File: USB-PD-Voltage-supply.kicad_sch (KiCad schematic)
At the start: 0 parts

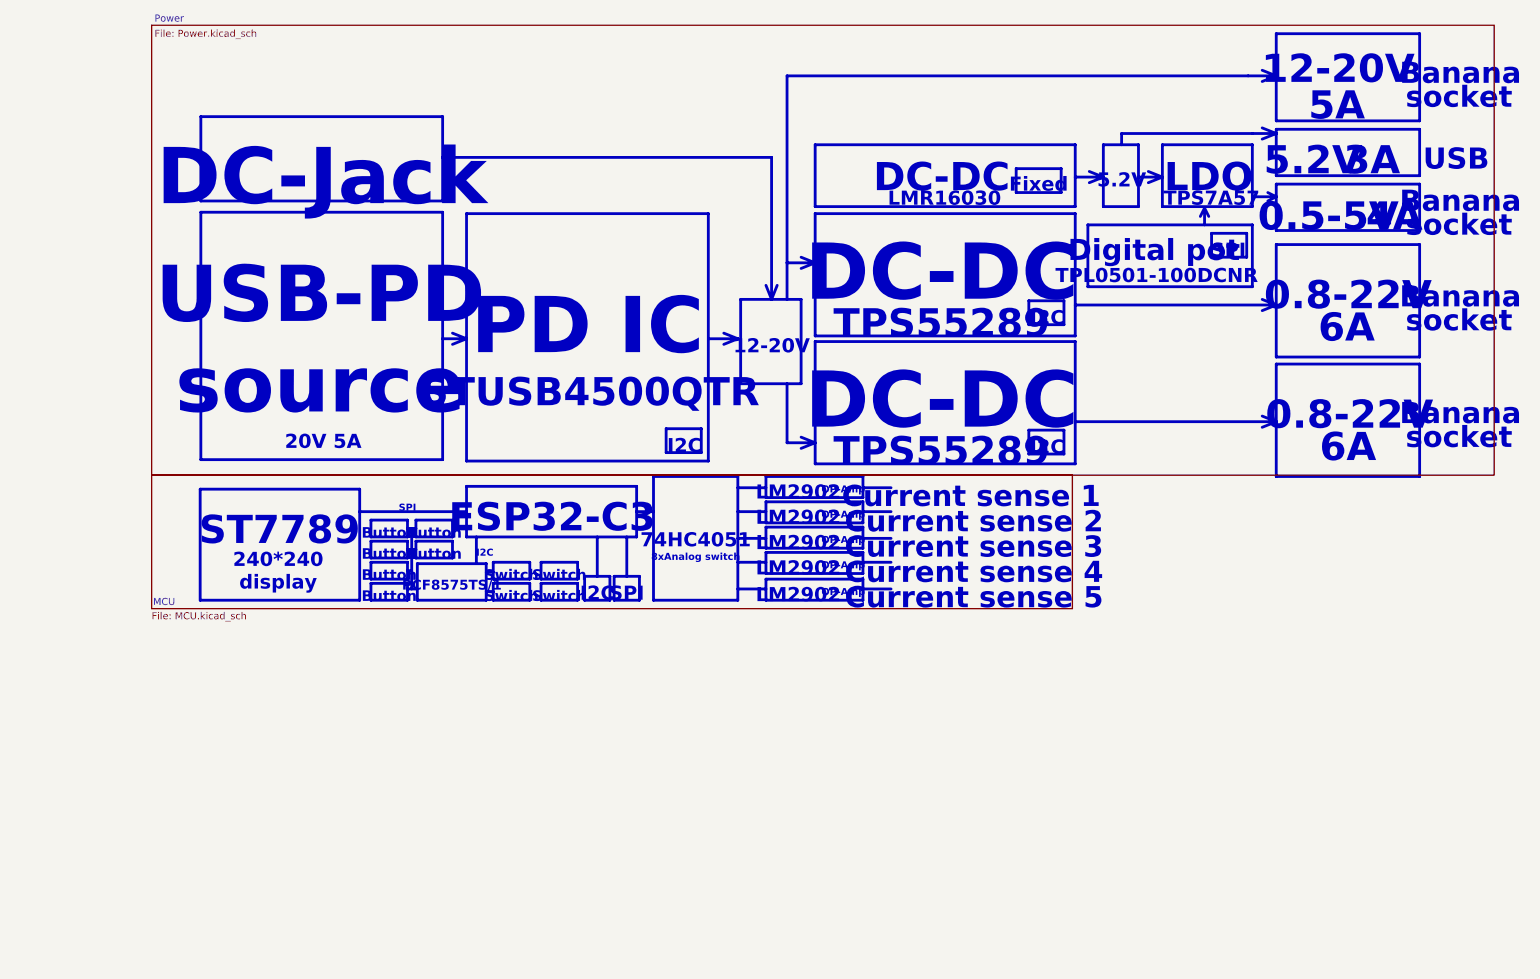
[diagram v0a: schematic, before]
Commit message: Почти завершённая схема
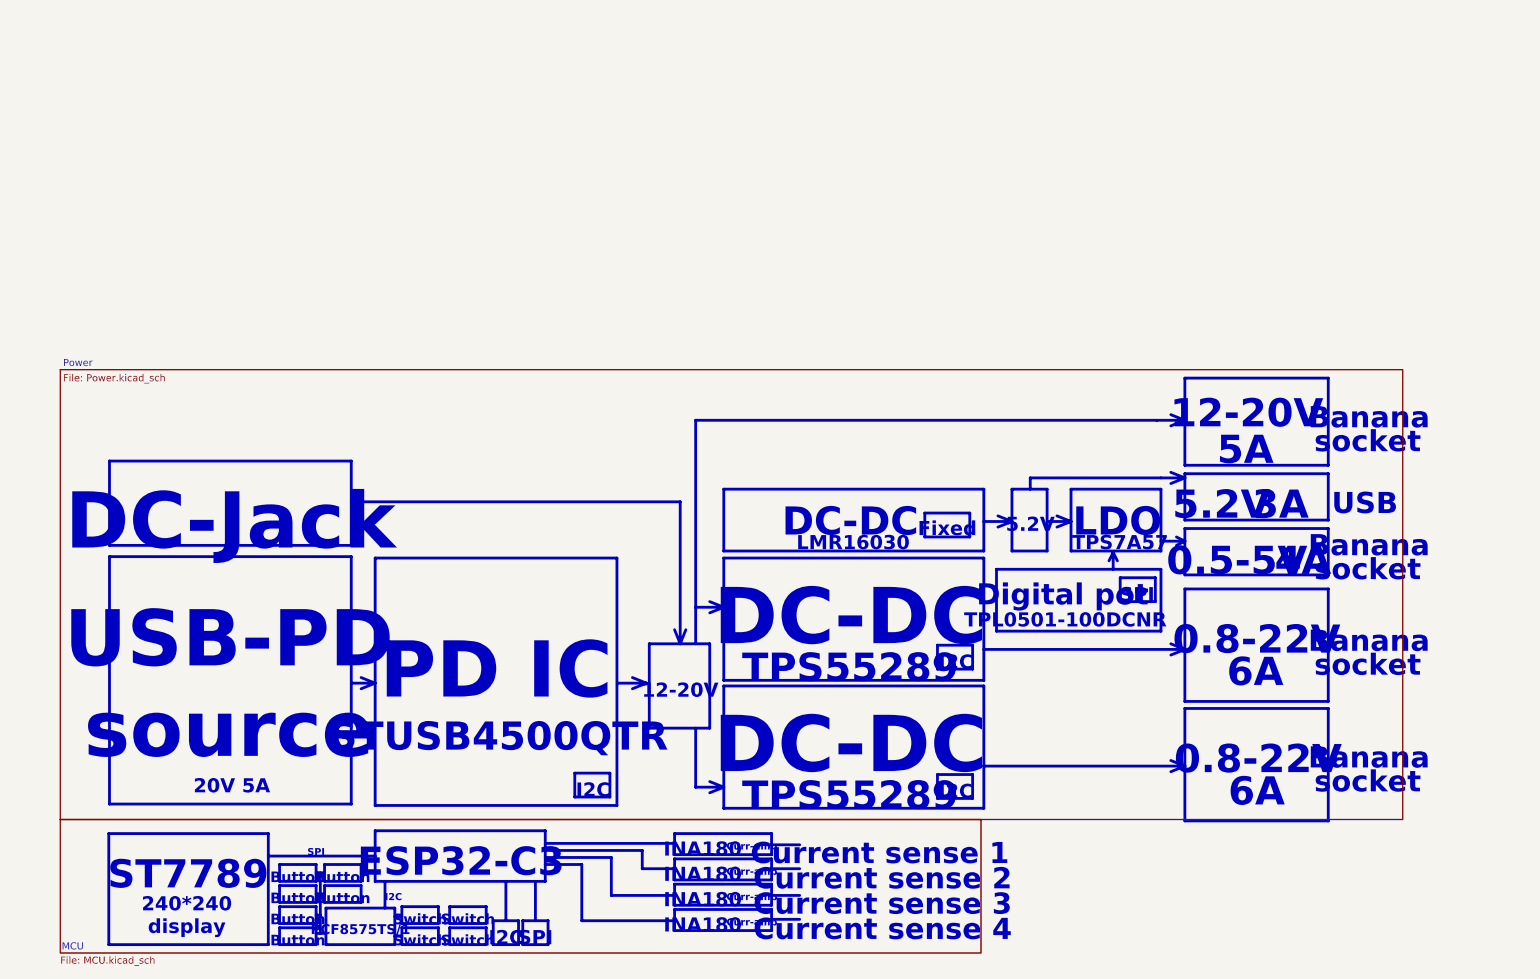
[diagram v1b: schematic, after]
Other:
- note added: "Curr-amp"
- note added: "INA180"
- note removed: "74HC4051"
- note removed: "8xAnalog switch"
- note removed: "Current sense 5"
- note removed: "LM2902"
- note removed: "OP-Amp"
